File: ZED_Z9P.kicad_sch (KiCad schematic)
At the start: 42 parts, among them IC2 ZED-F9P-05B, J4 SMA-J-P-X-RA-TH1, Q12 PMOS, Q2 MMBT3904LT1G, Q7 BC849, Q8 BC849, Q9 BC849, U14 TPS22946YZPR, U3 MCP6001-OT

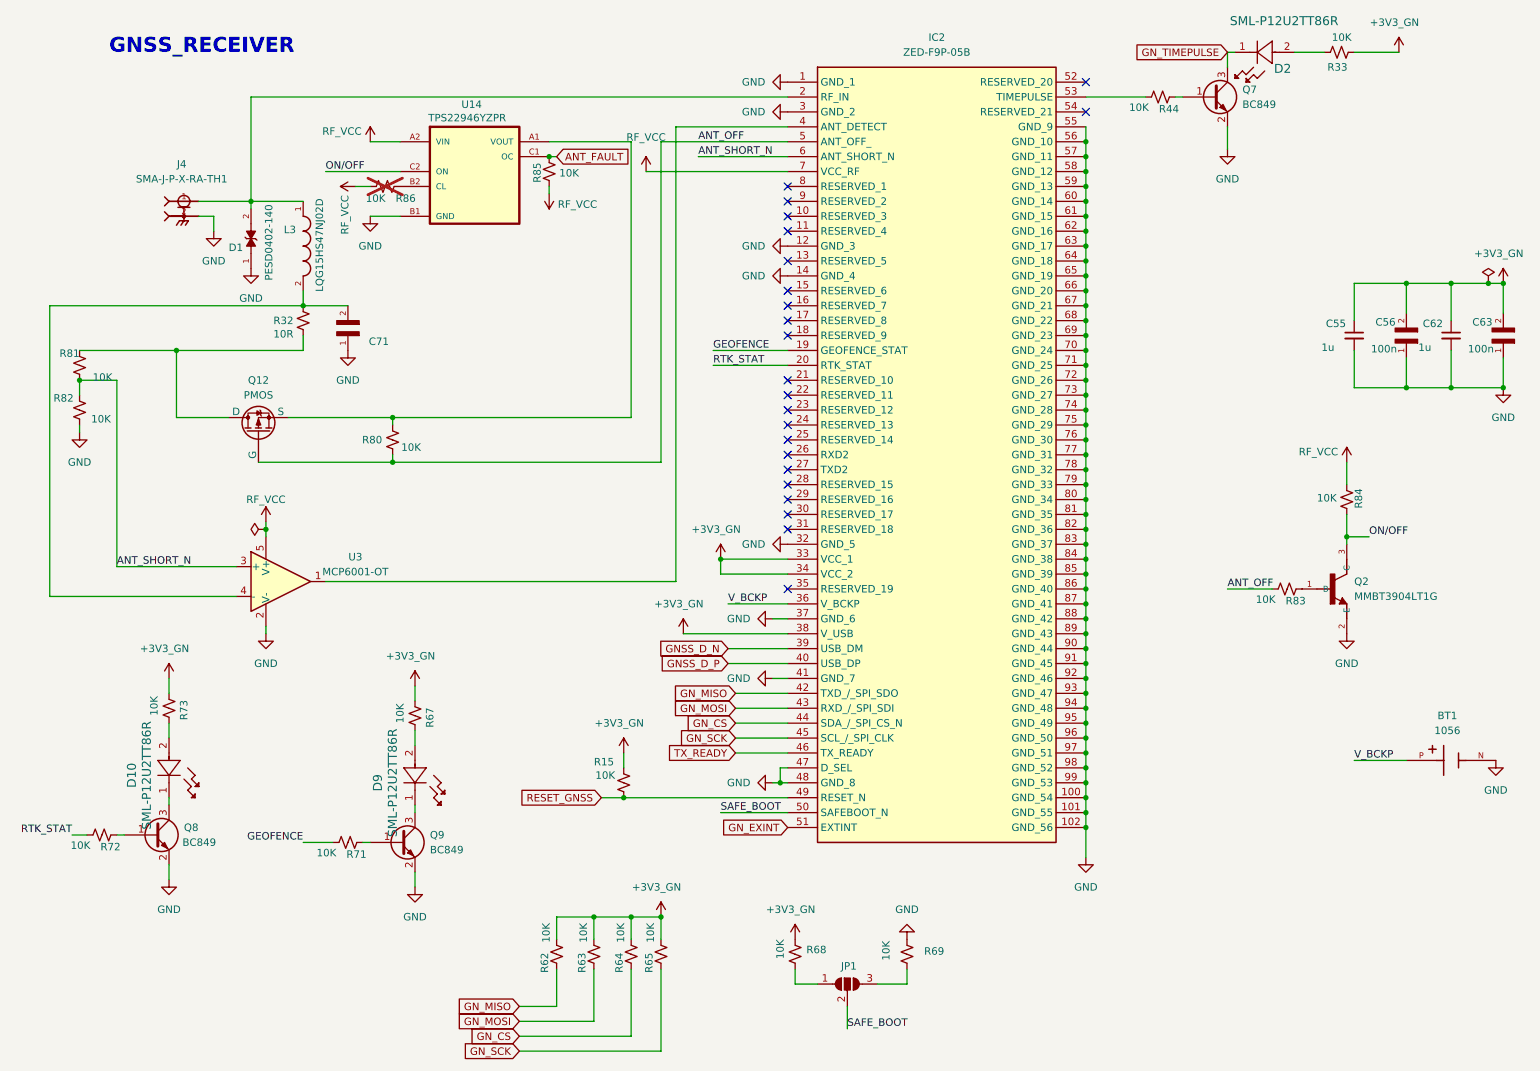
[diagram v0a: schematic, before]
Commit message: full
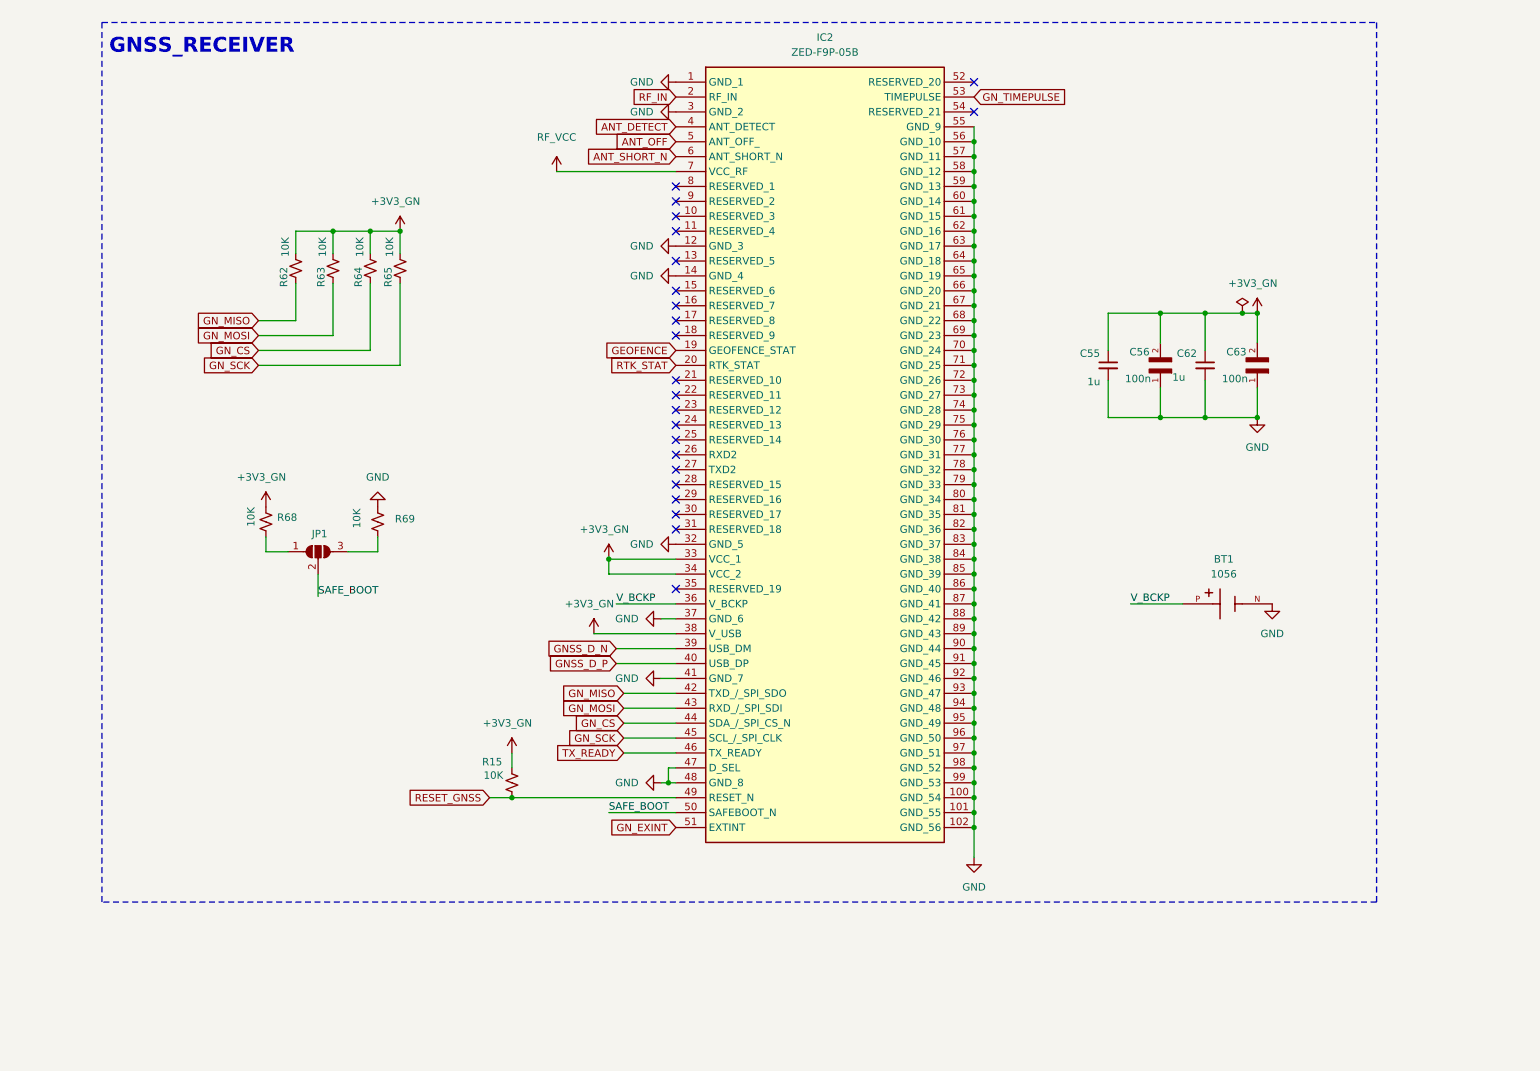
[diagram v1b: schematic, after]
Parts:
- removed C71: GRM033R71C103KE14D, GRM033R71C103KE14D:CAPC0603X33N, symbol GRM033R71C103KE14D:GRM033R71C103KE14D
- removed D1: PESD0402-140, PESD0402-140:DIO_PESD0402-140, symbol PESD0402-140:PESD0402-140
- removed D10, D2, D9: SML-P12U2TT86R, LED_SMD:LED_0402_1005Metric, symbol 2026-08-14_04-34-19:SML-P12U2TT86R
- removed J4: SMA-J-P-X-RA-TH1, GNSS:SAMTEC_SMA-J-P-X-RA-TH1, symbol SMA-J-P-X-RA-TH1:SMA-J-P-X-RA-TH1
- removed L3: LQG15HS47NJ02D, LQG15HS47NJ02D:INDC1005X55N, symbol LQG15HS47NJ02D:LQG15HS47NJ02D
- removed Q12: PMOS, symbol Simulation_SPICE:PMOS
- removed Q2: MMBT3904LT1G, MMBT3904LT1G:SOT95P240X111-3N, symbol MMBT3904LT1G:MMBT3904LT1G
- removed Q7, Q8, Q9: BC849, Package_TO_SOT_SMD:SOT-23, symbol Transistor_BJT:BC849
- removed R32: 10R, Resistor_SMD:R_0402_1005Metric, symbol Device:R_Small_US
- removed R33, R44, R67, R71, R72, R73, R80, R81, R82, R83, R84, R85, R86: 10K, Resistor_SMD:R_0402_1005Metric, symbol Device:R_Small_US
- removed U14: TPS22946YZPR, TPS22946YZPR:BGA6C50P2X3_140X90X50, symbol TPS22946YZPR:TPS22946YZPR
- removed U3: MCP6001-OT, Package_TO_SOT_SMD:SOT-23-5, symbol Amplifier_Operational:MCP6001-OT
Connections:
- net GN_TIMEPULSE: now also IC2.53 (TIMEPULSE)
- net RF_IN: now reaches IC2.2 (RF_IN)
- net ANT_DETECT: now reaches IC2.4 (ANT_DETECT)
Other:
- moved on the sheet: BT1, C55, C56, C62, C63, IC2, JP1, R15, R62, R63, R64, R65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
